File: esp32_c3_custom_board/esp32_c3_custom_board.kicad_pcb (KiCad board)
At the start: 2 copper layers, 44 parts, among them IC1 ESP32-C3, IC2 GD25Q16CTEGR, J1 USB-C Connector, U1 ESD Protection, U2 SPX3819M5-L-3-3, Y1 830108208709_crystal

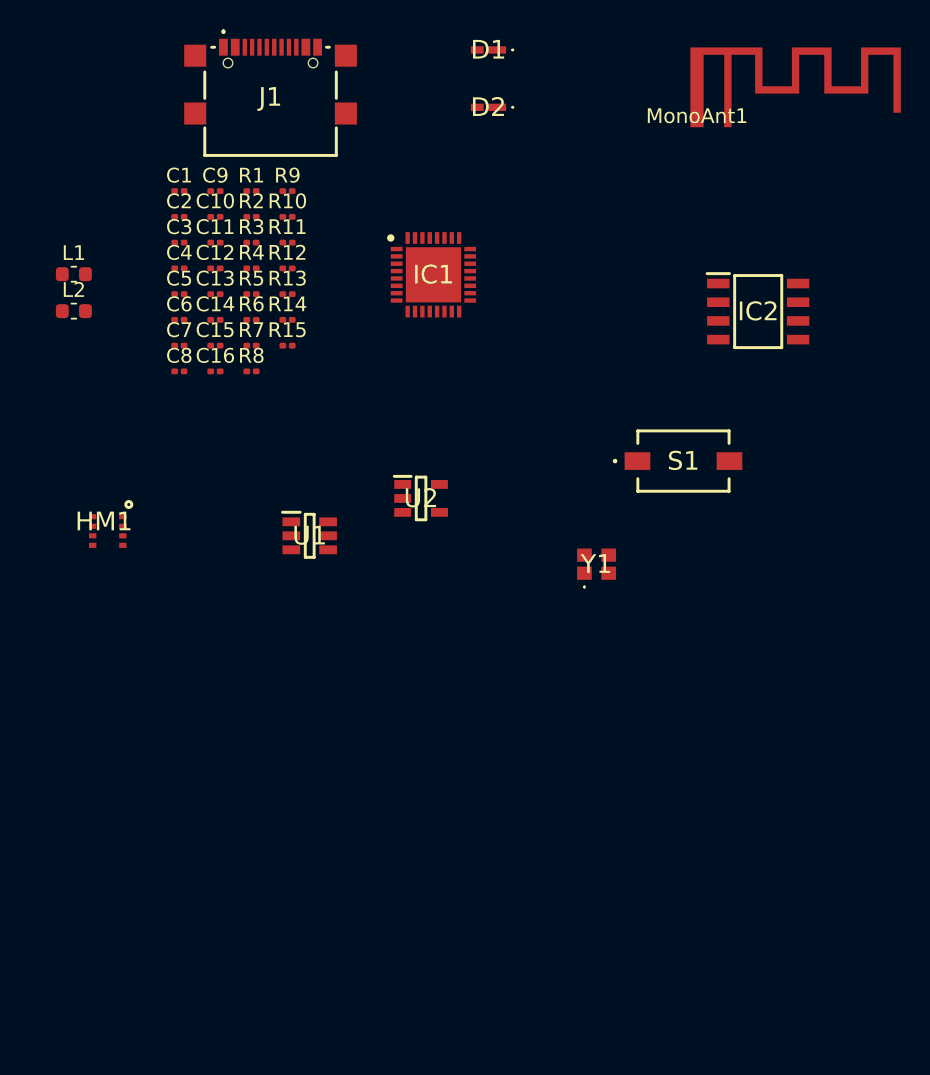
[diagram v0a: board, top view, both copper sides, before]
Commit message: .
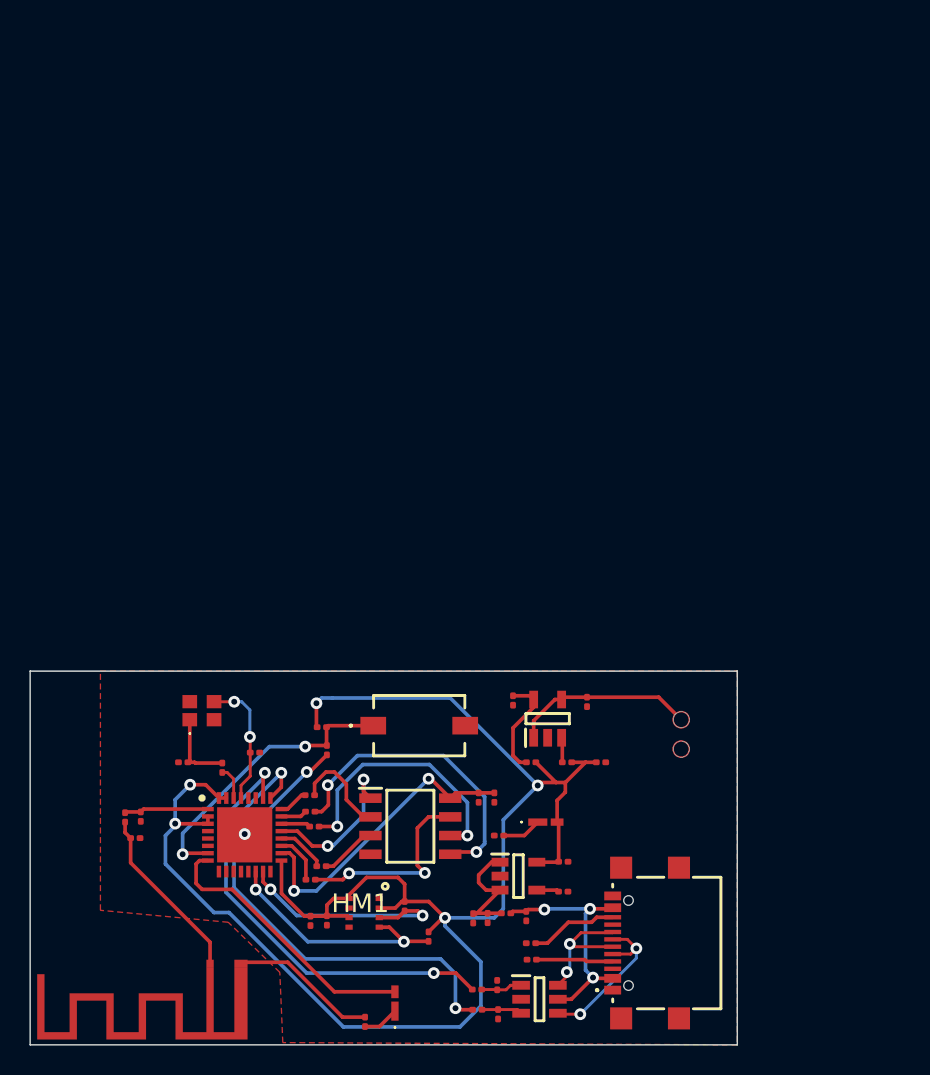
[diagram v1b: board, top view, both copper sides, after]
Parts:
- added C17: 22u, Capacitor_SMD:C_0201_0603Metric, F.Cu at (148.4, 133.2)
- added C18: 22u, Capacitor_SMD:C_0201_0603Metric, F.Cu at (149.3, 137.3)
- added IC3: SMD_IC_SY8089AAAC, SY8089AAAC:SOT95P285X140-5N, F.Cu at (145.7, 134.3)
- added JST1: ~, JST_Connectors:JST-PH2.0mm, F.Cu at (154.8, 134.4)
- added L3: 2.2u, Inductor_SMD:L_0201_0603Metric, F.Cu at (147.0, 137.3)
- added R16: 220k, Resistor_SMD:R_0201_0603Metric, F.Cu at (144.6, 137.3)
- added R17: 47k, Resistor_SMD:R_0201_0603Metric, F.Cu at (143.4, 133.1)
- L1, L2: footprint Inductor_SMD:L_0603_1608Metric -> Inductor_SMD:L_0201_0603Metric
- moved MonoAnt1 64.9 mm to (124.9, 151.0), turned to 180 degrees
- moved J1 63.4 mm to (153.5, 149.6), turned to 90 degrees
- moved D2 61.2 mm to (135.3, 153.7), turned to -90 degrees
- moved R9 54.8 mm to (144.6, 150.7), turned to 180 degrees
- moved C5 53.5 mm to (142.3, 154.4), turned to -90 degrees
- moved D1 52.6 mm to (145.6, 141.4), turned to 180 degrees
- moved C9 52.4 mm to (140.7, 147.9), turned to -90 degrees
- moved R10 52.1 mm to (144.6, 149.6)
- moved C10 52.0 mm to (144.3, 147.8), turned to -90 degrees
- moved L2 50.4 mm to (142.9, 147.6), turned to 180 degrees
- moved C6 50.1 mm to (142.3, 152.5), turned to 90 degrees
- moved R13 49.7 mm to (133.3, 155.0), turned to -90 degrees
- moved C11 49.5 mm to (141.6, 147.9), turned to -90 degrees
- moved R1 47.0 mm to (129.6, 145.3)
- moved R7 46.4 mm to (140.9, 152.8)
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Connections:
- C12 pad 2: unconnected-(C12-Pad2) -> GND
- IC1 pad 17: unconnected-(IC1-VDD3P3_CPU-Pad17) -> +3.3V
- IC1 pad 2: unconnected-(IC1-VDD3P3_1-Pad2) -> +3.3V
- IC1 pad 3: unconnected-(IC1-VDD3P3_2-Pad3) -> +3.3V
- IC1 pad 31: unconnected-(IC1-VDDA_1-Pad31) -> +3.3V
- IC1 pad 32: unconnected-(IC1-VDDA_2-Pad32) -> +3.3V
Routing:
- net +3.3V: track 0.00 -> 115.3 mm, vias 0 -> 5
- net Net-(IC1-GPIO18): track 0.00 -> 32.2 mm, vias 0 -> 2
- net Net-(IC1-GPIO19): track 0.00 -> 30.5 mm, vias 0 -> 2
- net /SPI_D: track 0.00 -> 20.9 mm, vias 0 -> 2
- net /VDD_SPI: track 0.00 -> 20.7 mm, vias 0 -> 2
- net Net-(IC1-CHIP_EN): track 0.00 -> 19.9 mm, vias 0 -> 2
- net /GPIO3: track 0.00 -> 18.8 mm
- net /SPI_CLK: track 0.00 -> 17.8 mm, vias 0 -> 2
- net GND: track 0.00 -> 17.7 mm, vias 0 -> 2
- net VBUS: track 0.00 -> 16.7 mm, vias 0 -> 3
- net /SCL: track 0.00 -> 16.5 mm, vias 0 -> 2
- net /SDA: track 0.00 -> 15.8 mm, vias 0 -> 2
- net /SPI_HD: track 0.00 -> 13.4 mm, vias 0 -> 2
- net Net-(IC3-EN): track 0.00 -> 12.5 mm
- net Net-(MonoAnt1-Feed): track 0.00 -> 11.9 mm
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- added copper zone on F.Cu, net GND
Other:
- board outline added: 48.1 x 25.4 mm
